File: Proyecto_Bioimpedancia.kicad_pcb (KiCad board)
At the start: 2 copper layers, 100 x 100 mm, 69 parts, among them J1 Jumper, J2 Jumper, J3 Jumper_Calibration, J4 Jumper, J5 Jumper, J6 Jumper, P1 SD_LAPIZ, P10 RS-232, P11 SOURCE_2, P12 RESET, P13 POWER, P14 BIO_OUT1, P15 GND_REGULATOR, P16 BIO_OUT2, P2 GPIO, P3 SOURCE_3, P4 SERIAL_VIRTUAL, P5 ENCODER, P6 I2C_1, P7 I2C_2, P8 SOURCE_1, P9 SPI, SW1 SW_PUSH, U1 AD8606, U2 ADG819, U3 Atmega328PA, U4 LD1117S50TR, Y1 XRCHA_16M

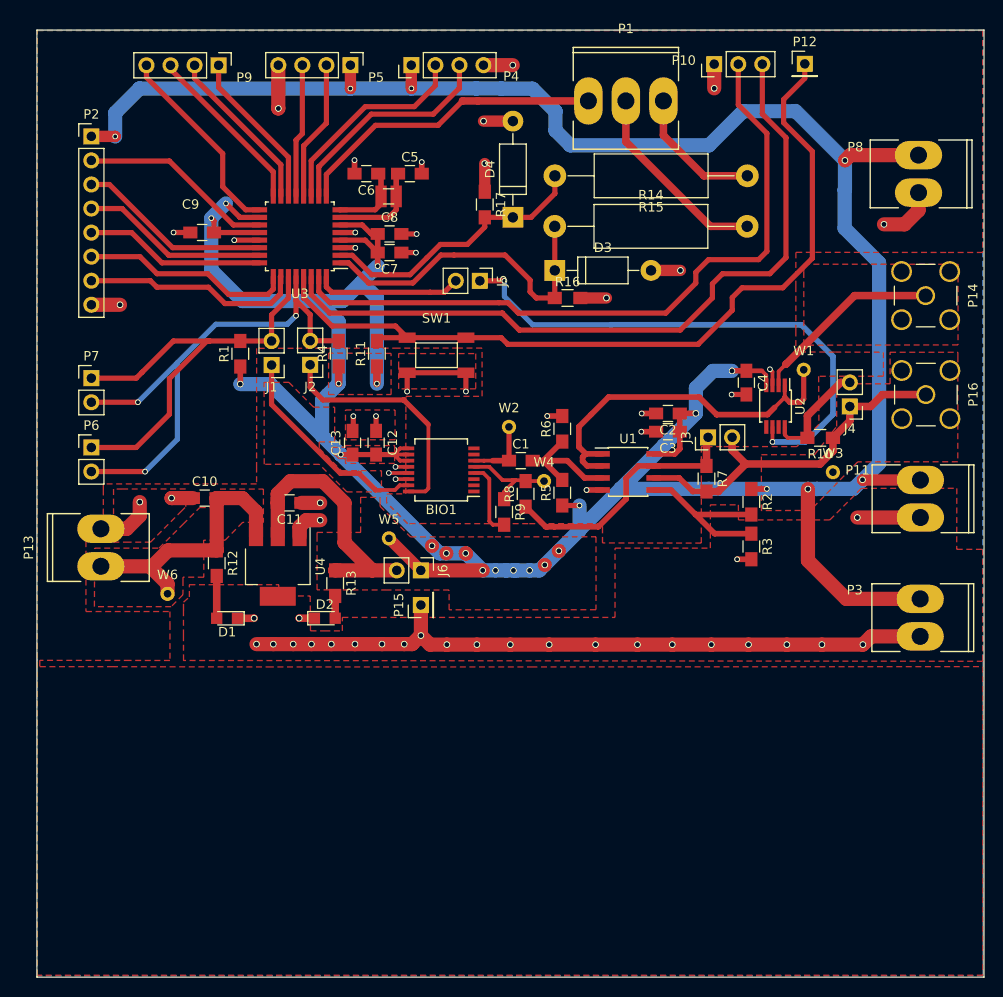
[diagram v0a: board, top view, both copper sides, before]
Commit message: PCB BIO mejorada con puertos I2C y capacitor para el puerto DTR del programador FTDI
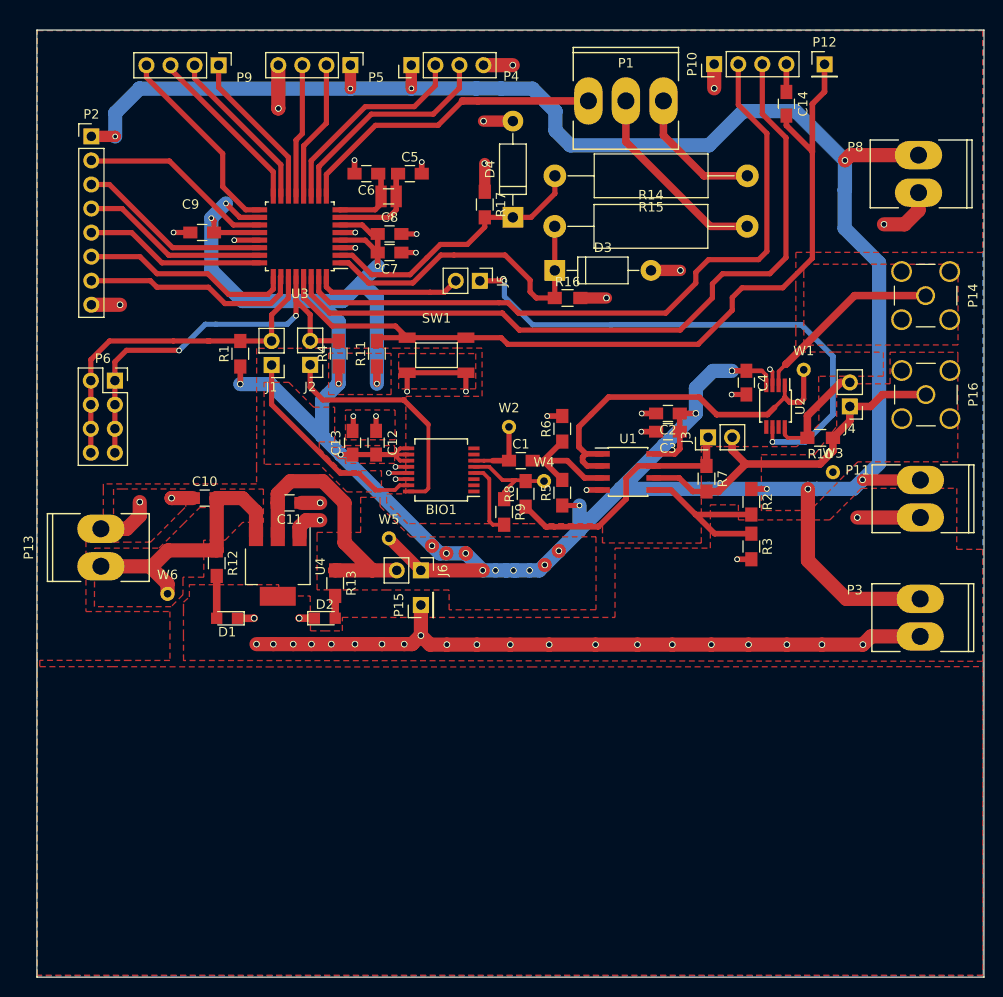
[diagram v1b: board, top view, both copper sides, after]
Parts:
- removed P7: I2C_2, Socket_Strips:Socket_Strip_Straight_1x02_Pitch2.54mm
- added C14: 0,1uF, Capacitors_SMD:C_0805_HandSoldering, F.Cu at (165.7, 53.0)
- P10: footprint Socket_Strips:Socket_Strip_Straight_1x03_Pitch2.54mm -> Socket_Strips:Socket_Strip_Straight_1x04_Pitch2.54mm
- P6: value I2C_1 -> CONN_02X04; footprint Socket_Strips:Socket_Strip_Straight_1x02_Pitch2.54mm -> Socket_Strips:Socket_Strip_Straight_2x04_Pitch2.54mm
- moved P6 7.49 mm to (94.8, 82.2)
- moved P12 2.09 mm to (169.7, 48.8)
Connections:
- P6 pad 1: /SDA_R -> /SCL_R
- P6 pad 2: /SCL_R -> /SDA_R
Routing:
- net /SCL_R: track 56.0 -> 42.8 mm, vias 3 -> 2
- net /SDA_R: track 47.7 -> 37.6 mm
- net /RESET: track 89.0 -> 92.3 mm
- net Net-(C14-Pad1): track 0.00 -> 2.94 mm

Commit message: Revert "PCB BIO mejorada con puertos I2C y capacitor para el puerto DTR del programador FTDI"
This reverts commit 0fb084b6cb4dcbd826a5771fbeb8258d6327cef0.
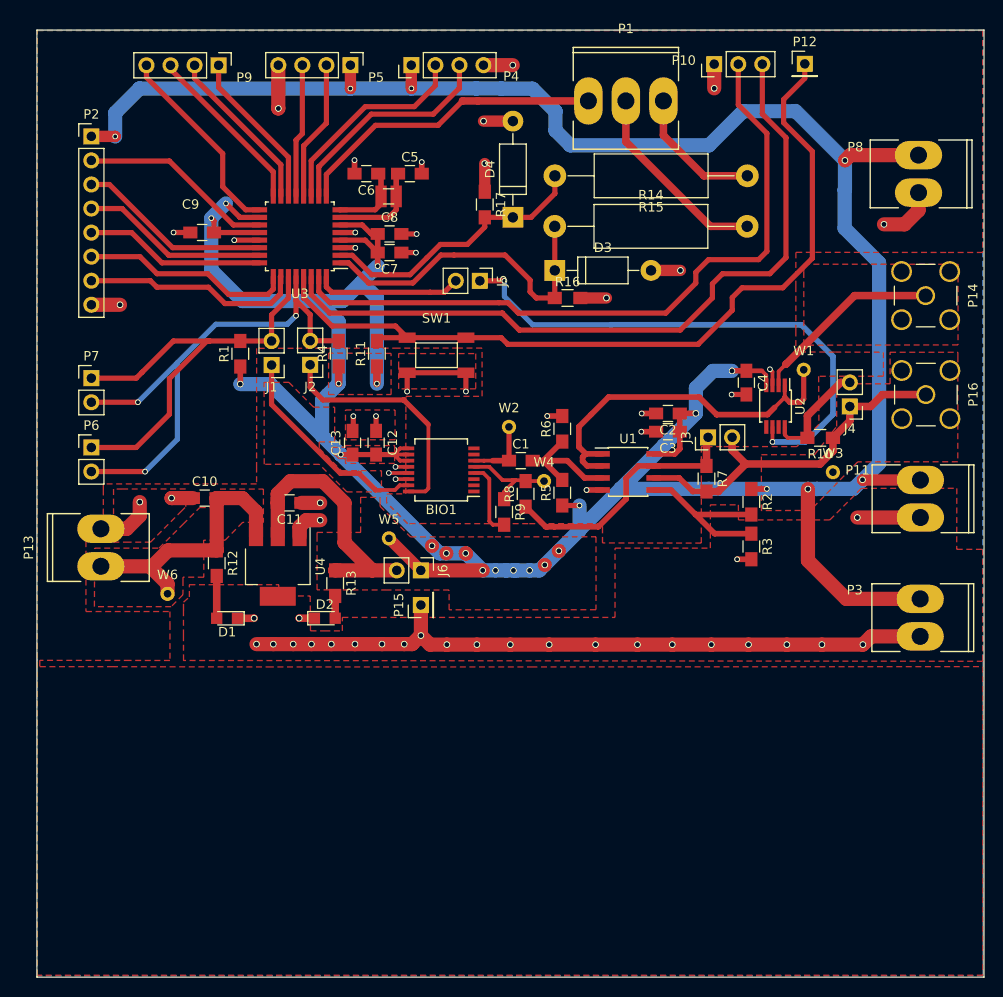
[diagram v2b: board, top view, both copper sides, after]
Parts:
- removed C14: 0,1uF, Capacitors_SMD:C_0805_HandSoldering
- added P7: I2C_2, Socket_Strips:Socket_Strip_Straight_1x02_Pitch2.54mm, F.Cu at (92.3, 82.0)
- P10: footprint Socket_Strips:Socket_Strip_Straight_1x04_Pitch2.54mm -> Socket_Strips:Socket_Strip_Straight_1x03_Pitch2.54mm
- P6: value CONN_02X04 -> I2C_1; footprint Socket_Strips:Socket_Strip_Straight_2x04_Pitch2.54mm -> Socket_Strips:Socket_Strip_Straight_1x02_Pitch2.54mm
- moved P6 7.49 mm to (92.3, 89.3)
- moved P12 2.09 mm to (167.6, 48.8)
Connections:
- P6 pad 1: /SCL_R -> /SDA_R
- P6 pad 2: /SDA_R -> /SCL_R
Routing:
- net /SCL_R: track 42.8 -> 56.0 mm, vias 2 -> 3
- net /SDA_R: track 37.6 -> 47.7 mm
- net /RESET: track 92.3 -> 89.0 mm
- net Net-(C14-Pad1): track 2.94 -> 0.00 mm
